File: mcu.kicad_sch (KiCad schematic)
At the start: 28 parts, among them J1 FTSH-105-01-F-DV-P-TR, J5 2337019-1, SW1 SW_Push, U1 nRF52840, U5 MX25R6435FZAIL0, U6 AP22814AW5, Y1 32MHz, Y2 32.768kHz

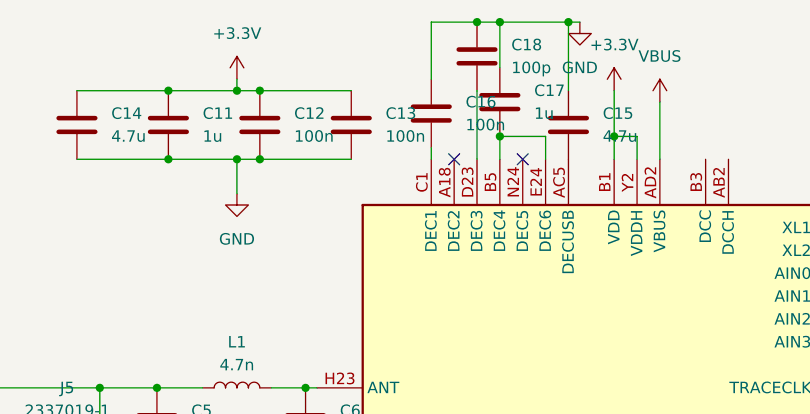
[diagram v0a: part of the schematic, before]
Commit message: finished schematic
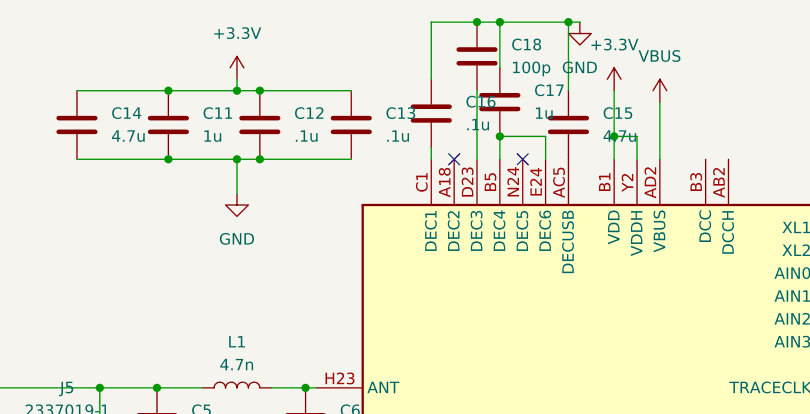
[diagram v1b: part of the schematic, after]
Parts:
- C1, C2, C3, C4: footprint (none) -> Capacitor_SMD:C_0603_1608Metric; LCSC PN (none) -> C107034
- C11, C17: footprint (none) -> Capacitor_SMD:C_0603_1608Metric; LCSC PN (none) -> C15849
- C12, C13, C16: value 100n -> .1u; footprint (none) -> Capacitor_SMD:C_0603_1608Metric; LCSC PN (none) -> C14663
- C14, C15: footprint (none) -> Capacitor_SMD:C_0603_1608Metric; LCSC PN (none) -> C19666
- C18: footprint (none) -> Capacitor_SMD:C_0603_1608Metric; LCSC PN (none) -> C14665
- C21, C22: footprint (none) -> Capacitor_SMD:C_0603_1608Metric; LCSC PN (none) -> C710896
- C5: footprint (none) -> Capacitor_SMD:C_0603_1608Metric; LCSC PN (none) -> C162254
- C6: footprint (none) -> Capacitor_SMD:C_0603_1608Metric; LCSC PN (none) -> C907996
- L1: footprint (none) -> Inductor_SMD:L_0603_1608Metric; LCSC PN (none) -> C98078
- L2: footprint (none) -> Inductor_SMD:L_0603_1608Metric; LCSC PN (none) -> C2042508
- R10: footprint (none) -> Resistor_SMD:R_0603_1608Metric; LCSC PN (none) -> C98220
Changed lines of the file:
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@@
 			)
 		)
-		(property "Footprint" ""
+		(property "Footprint" "Capacitor_SMD:C_0603_1608Metric"
 			(at 111.4552 20.32 0)
 			(effects
@@
 			)
 		)
+		(property "LCSC PN" "C14665"
+			(at 110.49 16.51 0)
+			(effects
+				(font
+					(size 1.27 1.27)
+				)
+				(hide yes)
+			)
+		)
 		(pin "2"
 		)
@@
 			)
 		)
-		(property "Footprint" ""
+		(property "Footprint" "Capacitor_SMD:C_0603_1608Metric"
 			(at 113.9952 25.4 0)
 			(effects
@@
 			)
 		)
+		(property "LCSC PN" "C15849"
+			(at 113.03 21.59 0)
+			(effects
+				(font
+					(size 1.27 1.27)
+				)
+				(hide yes)
+			)
+		)
 		(pin "2"
 		)
@@
 			)
 		)
-		(property "Value" "100n"
+		(property "Value" ".1u"
 			(at 100.33 25.3999 0)
 			(effects
@@
 			)
 		)
-		(property "Footprint" ""
+		(property "Footprint" "Capacitor_SMD:C_0603_1608Metric"
 			(at 97.4852 27.94 0)
 			(effects
@@
 			)
 		)
+		(property "LCSC PN" "C14663"
+			(at 96.52 24.13 0)
+			(effects
+				(font
+					(size 1.27 1.27)
+				)
+				(hide yes)
+			)
+		)
 		(pin "2"
 		)
@@
 			)
 		)
-		(property "Footprint" ""
+		(property "Footprint" "Capacitor_SMD:C_0603_1608Metric"
 			(at 72.39 103.1748 0)
 			(effects
@@
 			)
 		)
+		(property "LCSC PN" "C107034"
+			(at 68.58 104.14 90)
+			(effects
+				(font
+					(size 1.27 1.27)
+				)
+				(hide yes)
+			)
+		)
 		(pin "2"
 		)
@@
 			)
 		)
-		(property "Footprint" ""
+		(property "Footprint" "Capacitor_SMD:C_0603_1608Metric"
 			(at 75.8952 60.96 0)
 			(effects
@@
 			)
 		)
+		(property "LCSC PN" "C162254"
+			(at 74.93 57.15 0)
+			(effects
+				(font
+					(size 1.27 1.27)
+				)
+				(hide yes)
+			)
+		)
 		(pin "2"
 		)
@@
 			)
 		)
-		(property "Footprint" ""
+		(property "Footprint" "Inductor_SMD:L_0603_1608Metric"
 			(at 40.64 53.34 0)
 			(effects
@@
 			)
 		)
+		(property "LCSC PN" "C2042508"
+			(at 40.64 53.34 90)
+			(effects
+				(font
+					(size 1.27 1.27)
+				)
+				(hide yes)
+			)
+		)
 		(pin "2"
 		)
@@
 			)
 		)
-		(property "Value" "100n"
+		(property "Value" ".1u"
 			(at 109.22 24.1299 0)
 			(effects
@@
 			)
 		)
-		(property "Footprint" ""
+		(property "Footprint" "Capacitor_SMD:C_0603_1608Metric"
 			(at 106.3752 26.67 0)
 			(effects
@@
 			)
 		)
+		(property "LCSC PN" "C14663"
+			(at 105.41 22.86 0)
+			(effects
+				(font
+					(size 1.27 1.27)
+				)
+				(hide yes)
+			)
+		)
 		(pin "2"
 		)
@@
 			)
 		)
-		(property "Footprint" ""
+		(property "Footprint" "Capacitor_SMD:C_0603_1608Metric"
 			(at 32.7152 60.96 0)
 			(effects
@@
 			)
 		)
+		(property "LCSC PN" "C710896"
+			(at 31.75 57.15 0)
+			(effects
+				(font
+					(size 1.27 1.27)
+				)
+				(hide yes)
+			)
+		)
 		(pin "2"
 		)
@@
 			)
 		)
-		(property "Footprint" ""
+		(property "Footprint" "Capacitor_SMD:C_0603_1608Metric"
 			(at 77.1652 27.94 0)
 			(effects
@@
 			)
 		)
+		(property "LCSC PN" "C15849"
+			(at 76.2 24.13 0)
+			(effects
+				(font
+					(size 1.27 1.27)
+				)
+				(hide yes)
+			)
+		)
 		(pin "2"
 		)
@@
 			)
 		)
-		(property "Footprint" ""
+		(property "Footprint" "Inductor_SMD:L_0603_1608Metric"
 			(at 83.82 53.34 0)
 			(effects
@@
 			)
 		)
+		(property "LCSC PN" "C98078"
+			(at 83.82 53.34 90)
+			(effects
+				(font
+					(size 1.27 1.27)
+				)
+				(hide yes)
+			)
+		)
 		(pin "2"
 		)
@@
 			)
 		)
-		(property "Footprint" ""
+		(property "Footprint" "Capacitor_SMD:C_0603_1608Metric"
 			(at 119.6848 20.32 0)
 			(effects
@@
 			)
 		)
+		(property "LCSC PN" "C19666"
+			(at 120.65 24.13 0)
+			(effects
+				(font
+					(size 1.27 1.27)
+				)
+				(hide yes)
+			)
+		)
 		(pin "2"
 		)
@@
 			)
 		)
-		(property "Footprint" ""
+		(property "Footprint" "Capacitor_SMD:C_0603_1608Metric"
 			(at 203.2 32.0548 0)
 			(effects
@@
 			)
 		)
+		(property "LCSC PN" "C107034"
+			(at 199.39 33.02 90)
+			(effects
+				(font
+					(size 1.27 1.27)
+				)
+				(hide yes)
+			)
+		)
 		(pin "2"
 		)
@@
 			)
 		)
-		(property "Footprint" ""
+		(property "Footprint" "Capacitor_SMD:C_0603_1608Metric"
 			(at 92.4052 60.96 0)
 			(effects
@@
 			)
 		)
+		(property "LCSC PN" "C907996"
+			(at 91.44 57.15 0)
+			(effects
+				(font
+					(size 1.27 1.27)
+				)
+				(hide yes)
+			)
+		)
 		(pin "1"
 		)
@@
 			)
 		)
-		(property "Footprint" ""
+		(property "Footprint" "Resistor_SMD:R_0603_1608Metric"
 			(at 235.712 45.72 90)
 			(effects
@@
 			)
 		)
+		(property "LCSC PN" "C98220"
+			(at 237.49 45.72 0)
+			(effects
+				(font
+					(size 1.27 1.27)
+				)
+				(hide yes)
+			)
+		)
 		(pin "1"
 		)
@@
 			)
 		)
-		(property "Footprint" ""
+		(property "Footprint" "Capacitor_SMD:C_0603_1608Metric"
 			(at 203.2 39.6748 0)
 			(effects
@@
 			)
 		)
+		(property "LCSC PN" "C107034"
+			(at 199.39 40.64 90)
+			(effects
+				(font
+					(size 1.27 1.27)
+				)
+				(hide yes)
+			)
+		)
 		(pin "1"
 		)
@@
 			)
 		)
-		(property "Footprint" ""
+		(property "Footprint" "Capacitor_SMD:C_0603_1608Metric"
 			(at 67.0052 27.94 0)
 			(effects
@@
 			)
 		)
+		(property "LCSC PN" "C19666"
+			(at 66.04 24.13 0)
+			(effects
+				(font
+					(size 1.27 1.27)
+				)
+				(hide yes)
+			)
+		)
 		(pin "2"
 		)
@@
 			)
 		)
-		(property "Footprint" ""
+		(property "Footprint" "Capacitor_SMD:C_0603_1608Metric"
 			(at 73.66 93.0148 0)
 			(effects
@@
 			)
 		)
+		(property "LCSC PN" "C107034"
+			(at 69.85 93.98 90)
+			(effects
+				(font
+					(size 1.27 1.27)
+				)
+				(hide yes)
+			)
+		)
 		(pin "1"
 		)
@@
 			)
 		)
-		(property "Footprint" ""
+		(property "Footprint" "Capacitor_SMD:C_0603_1608Metric"
 			(at 49.2252 60.96 0)
 			(effects
@@
 			)
 		)
+		(property "LCSC PN" "C710896"
+			(at 48.26 57.15 0)
+			(effects
+				(font
+					(size 1.27 1.27)
+				)
+				(hide yes)
+			)
+		)
 		(pin "1"
 		)
@@
 			)
 		)
-		(property "Value" "100n"
+		(property "Value" ".1u"
 			(at 90.17 25.3999 0)
 			(effects
@@
 			)
 		)
-		(property "Footprint" ""
+		(property "Footprint" "Capacitor_SMD:C_0603_1608Metric"
 			(at 87.3252 27.94 0)
 			(effects
@@
 			(at 86.36 24.13 0)
 			(effects
+				(font
+					(size 1.27 1.27)
+				)
+				(hide yes)
+			)
+		)
+		(property "LCSC PN" "C14663"
+			(at 86.36 24.13 0)
+			(effects

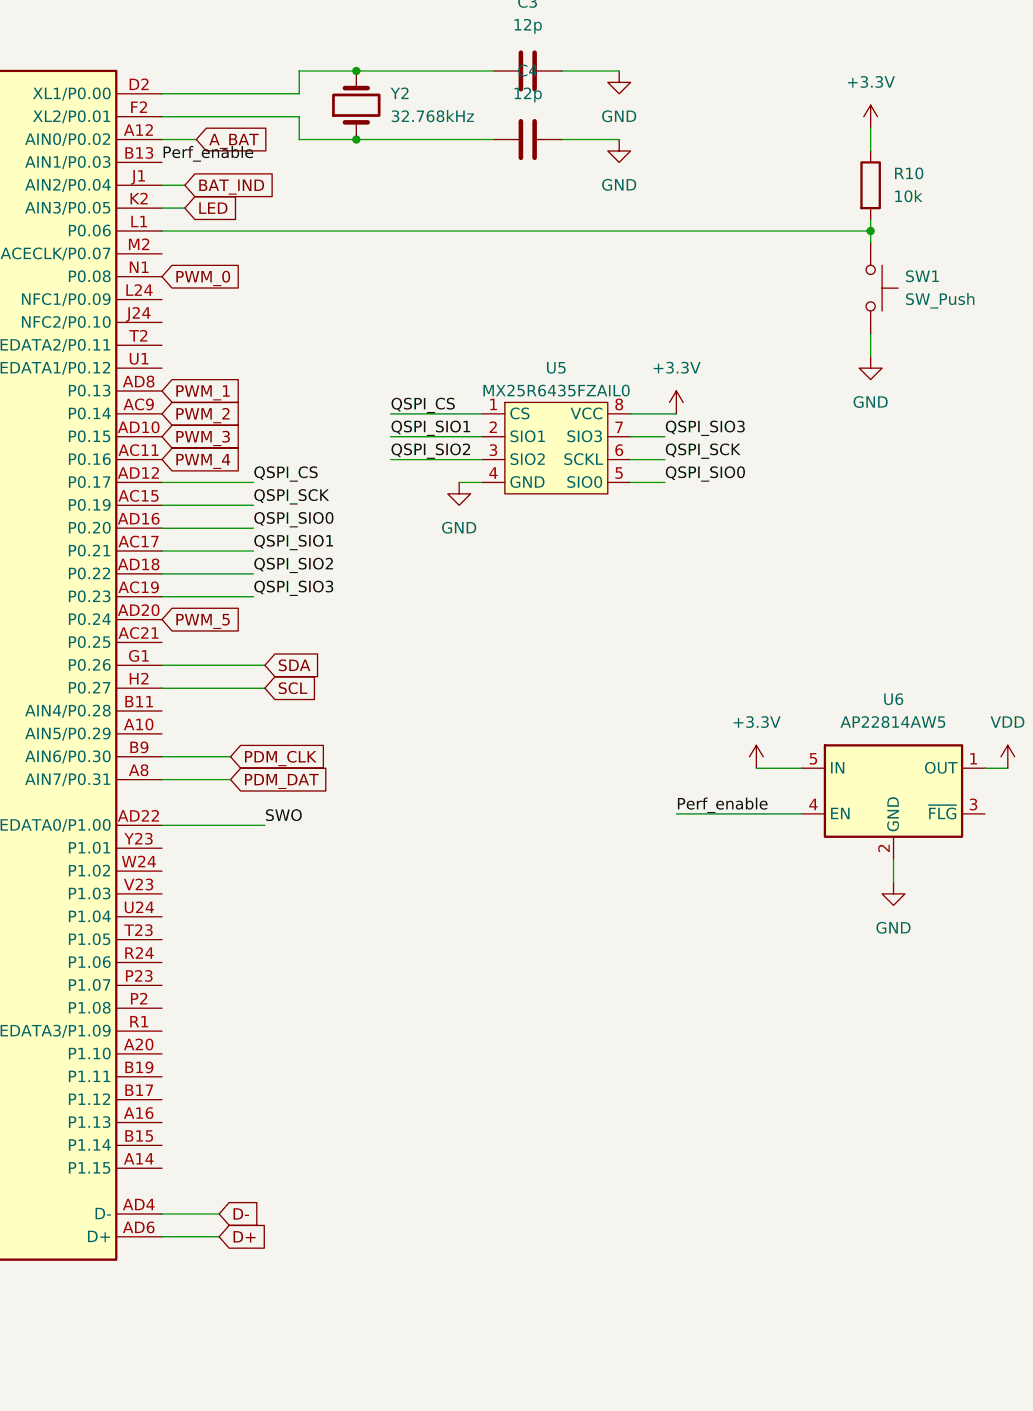
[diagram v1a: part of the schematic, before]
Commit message: PCB layout
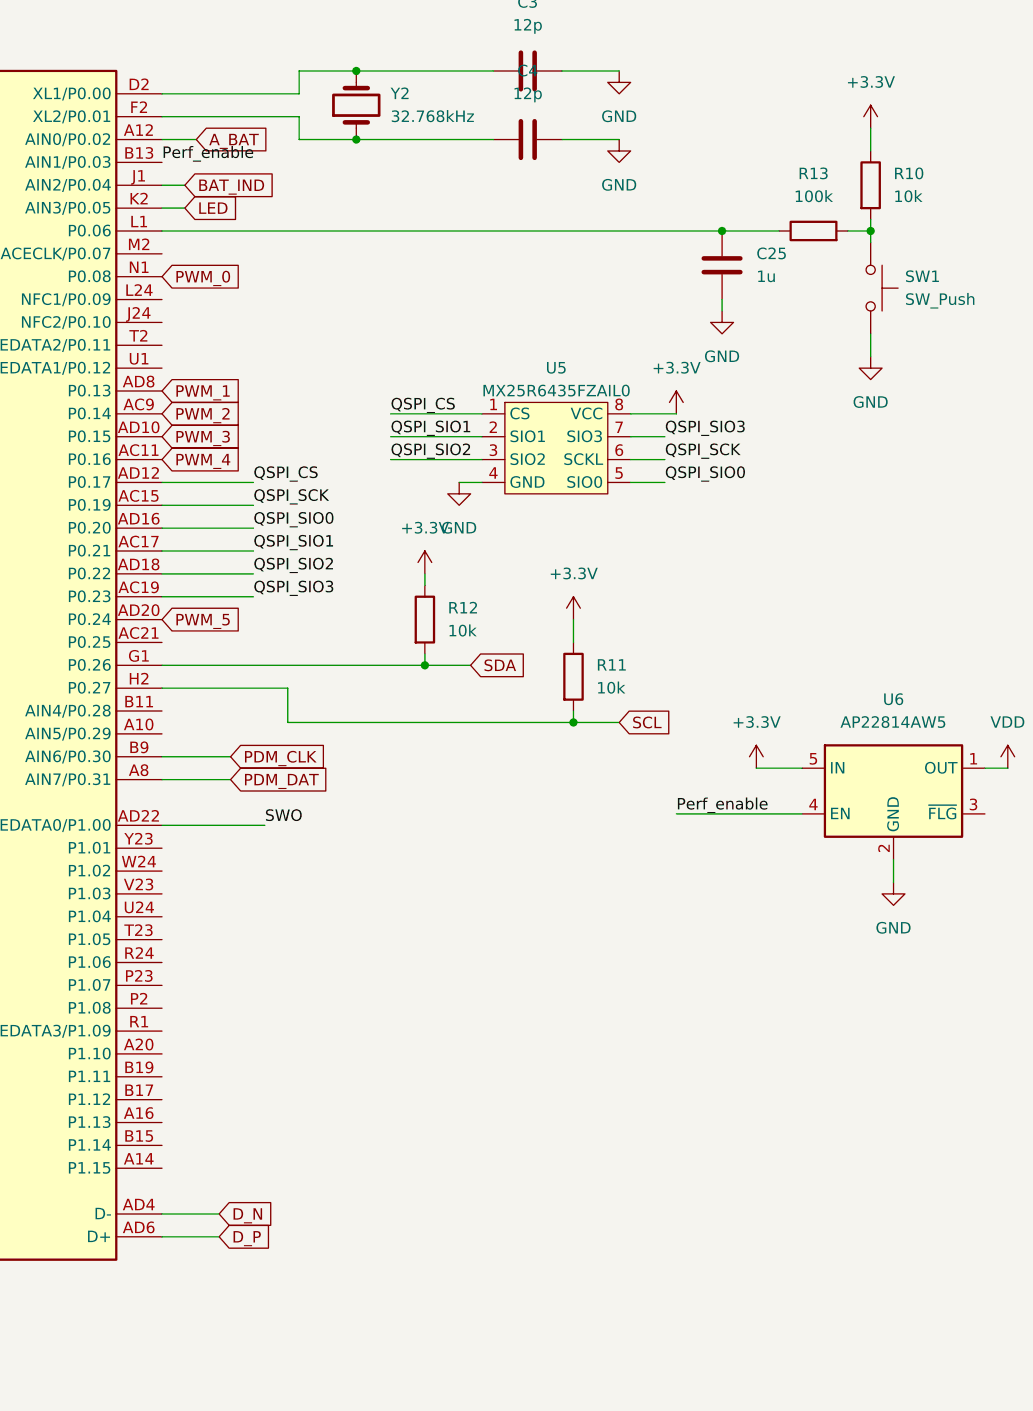
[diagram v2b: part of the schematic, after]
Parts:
- added C25: 1u, Capacitor_SMD:C_0603_1608Metric, symbol Device:C
- added R11, R12: 10k, Resistor_SMD:R_0603_1608Metric, symbol Device:R
- added R13: 100k, Resistor_SMD:R_0603_1608Metric, symbol Device:R
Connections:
- net +3.3V: now also R11.1, R12.1
- net GND: now also C25.2
- net SCL: now also R11.2
- net SDA: now also R12.2
- net at R10.2, SW1.1: now also R13.2; no longer U1.L1 (P0.06)
- net D+ renamed D_P
- net D- renamed D_N
- new net: C25.1, R13.1, U1.L1 (P0.06)
